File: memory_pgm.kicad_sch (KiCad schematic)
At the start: 14 parts

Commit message: Switch ROM chips to SRAM and add onboard programmer
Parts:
- removed J?: Conn_02x20_Odd_Even, symbol Connector_Generic:Conn_02x20_Odd_Even
- removed U? (x2): 28C256, symbol Memory_EEPROM:28C256
- removed U? (x4): 74HC245, symbol 74xx:74HC245
- removed U? (x5): 74LS32, symbol 74xx:74LS32
- added D? (x3): 1N4148, Diode_THT:D_DO-35_SOD27_P7.62mm_Horizontal, symbol Diode:1N4148
- added J?: QT Py RP2040, symbol Connector_Generic:Conn_02x07_Counter_Clockwise
- added J?: QT Py Serial, symbol Connector_Generic:Conn_01x03
- added R? (x6): 10K, symbol Device:R_Small_US
- added U? (x4): HEF4094BT, symbol parts:HEF4094BT
- added U? (x2): CY62256-70PC, Package_DIP:DIP-28_W15.24mm, symbol Memory_RAM:CY62256-70PC
- added U?: 74LS243, symbol 74xx:74LS243
- added U?: TXB0104PW, Package_SO:TSSOP-14_4.4x5mm_P0.65mm, symbol Logic_LevelTranslator:TXB0104PW
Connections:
- net A1: now also U?.10 (A0), U?.10 (A0), U?.4 (QP0)
- net A10: now also U?.24 (A9), U?.24 (A9), U?.5 (QP1)
- net A11: now also U?.21 (A10), U?.21 (A10), U?.6 (QP2)
- net A12: now also U?.23 (A11), U?.23 (A11), U?.7 (QP3)
- net A13: now also U?.14 (QP4), U?.2 (A12), U?.2 (A12)
- net A14: now also U?.13 (QP5), U?.26 (A13), U?.26 (A13)
- net A2: now also U?.5 (QP1), U?.9 (A1), U?.9 (A1)
- net A3: now also U?.6 (QP2), U?.8 (A2), U?.8 (A2)
- net A4: now also U?.7 (A3), U?.7 (A3), U?.7 (QP3)
- net A5: now also U?.14 (QP4), U?.6 (A4), U?.6 (A4)
- net A6: now also U?.13 (QP5), U?.5 (A5), U?.5 (A5)
- net A7: now also U?.12 (QP6), U?.4 (A6), U?.4 (A6)
- net A8: now also U?.11 (QP7), U?.3 (A7), U?.3 (A7)
- net A9: now also U?.25 (A8), U?.25 (A8), U?.4 (QP0)
- net D0: now also U?.11 (Q0), U?.4 (QP0)
- net D1: now also U?.12 (Q1), U?.5 (QP1)
- net D10: now also U?.13 (Q2), U?.6 (QP2)
- net D11: now also U?.15 (Q3), U?.7 (QP3)
- net D12: now also U?.14 (QP4), U?.16 (Q4)
- net D13: now also U?.13 (QP5), U?.17 (Q5)
- net D14: now also U?.12 (QP6), U?.18 (Q6)
- net D15: now also U?.11 (QP7), U?.19 (Q7)
- net D2: now also U?.13 (Q2), U?.6 (QP2)
- net D3: now also U?.15 (Q3), U?.7 (QP3)
- net D4: now also U?.14 (QP4), U?.16 (Q4)
- net D5: now also U?.13 (QP5), U?.17 (Q5)
- net D6: now also U?.12 (QP6), U?.18 (Q6)
- net D7: now also U?.11 (QP7), U?.19 (Q7)
- net D8: now also U?.11 (Q0), U?.4 (QP0)
- net D9: now also U?.12 (Q1), U?.5 (QP1)
- net GND: now also J?.13 (Pin_13), J?.3 (Pin_3), U?.1 (A14), U?.1 (A14), U?.14 (GND), U?.14 (GND), U?.5 (A4), U?.7 (GND), U?.7 (GND), U?.8 (B3), U?.8 (Vss), U?.8 (Vss), U?.8 (Vss), U?.8 (Vss)
- net VCC: now also R?.1, R?.1, R?.1, R?.1, R?.2, R?.2, U?.1 (OEa), U?.1 (STR), U?.1 (STR), U?.1 (STR), U?.1 (STR), U?.14 (VCC), U?.14 (VCCB), U?.16 (Vdd), U?.16 (Vdd), U?.16 (Vdd), U?.16 (Vdd), U?.28 (VCC), U?.28 (VCC)
- net ~{OE}: now also U?.22 (~{OE}), U?.22 (~{OE})
- net ~{ROMLDS}: now also U?.9 (B2)
- net ~{ROMUDS}: now also U?.10 (B1)
- net ~{WE}: now also U?.11 (B0); no longer U?.27 (~{WE}), U?.27 (~{WE})
- new net: R?.2, U?.12 (B2), U?.3 (CP), U?.3 (CP), U?.3 (CP), U?.3 (CP)
- new net: U?.10 (QS2), U?.2 (D) (x3)
- new net: D?.1 (K), D?.1 (K), D?.1 (K), R?.2, U?.10 (B4), U?.15 (~{OE}), U?.15 (~{OE}), U?.15 (~{OE}), U?.15 (~{OE})
- new net: J?.1 (Pin_1), U?.8 (OE)
- new net: J?.2 (Pin_2), U?.2 (A1)
- new net: J?.3 (Pin_3), U?.3 (A2)
- new net: J?.4 (Pin_4), U?.4 (A3)
- new net: J?.1 (Pin_1), J?.7 (Pin_7)
- new net: J?.2 (Pin_2), J?.8 (Pin_8)
- new net: R?.2, U?.13 (B1), U?.2 (D)
- new net +3V3: J?.12 (Pin_12), U?.1 (VCCA)
- new net ~{RESET}: D?.2 (A), U?.13 (OEb)
- new net ~{ROMLDS_INT}: D?.2 (A), R?.1, U?.20 (~{CS}), U?.5 (A2)
- new net ~{ROMUDS_INT}: D?.2 (A), R?.1, U?.20 (~{CS}), U?.4 (A1)
- new net ~{WE_INT}: R?.2, U?.11 (B3), U?.27 (~{WE}), U?.27 (~{WE}), U?.27 (~{WE}), U?.27 (~{WE}), U?.3 (A0)
- no-connect marks 2 -> 14
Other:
- moved on the sheet: U?

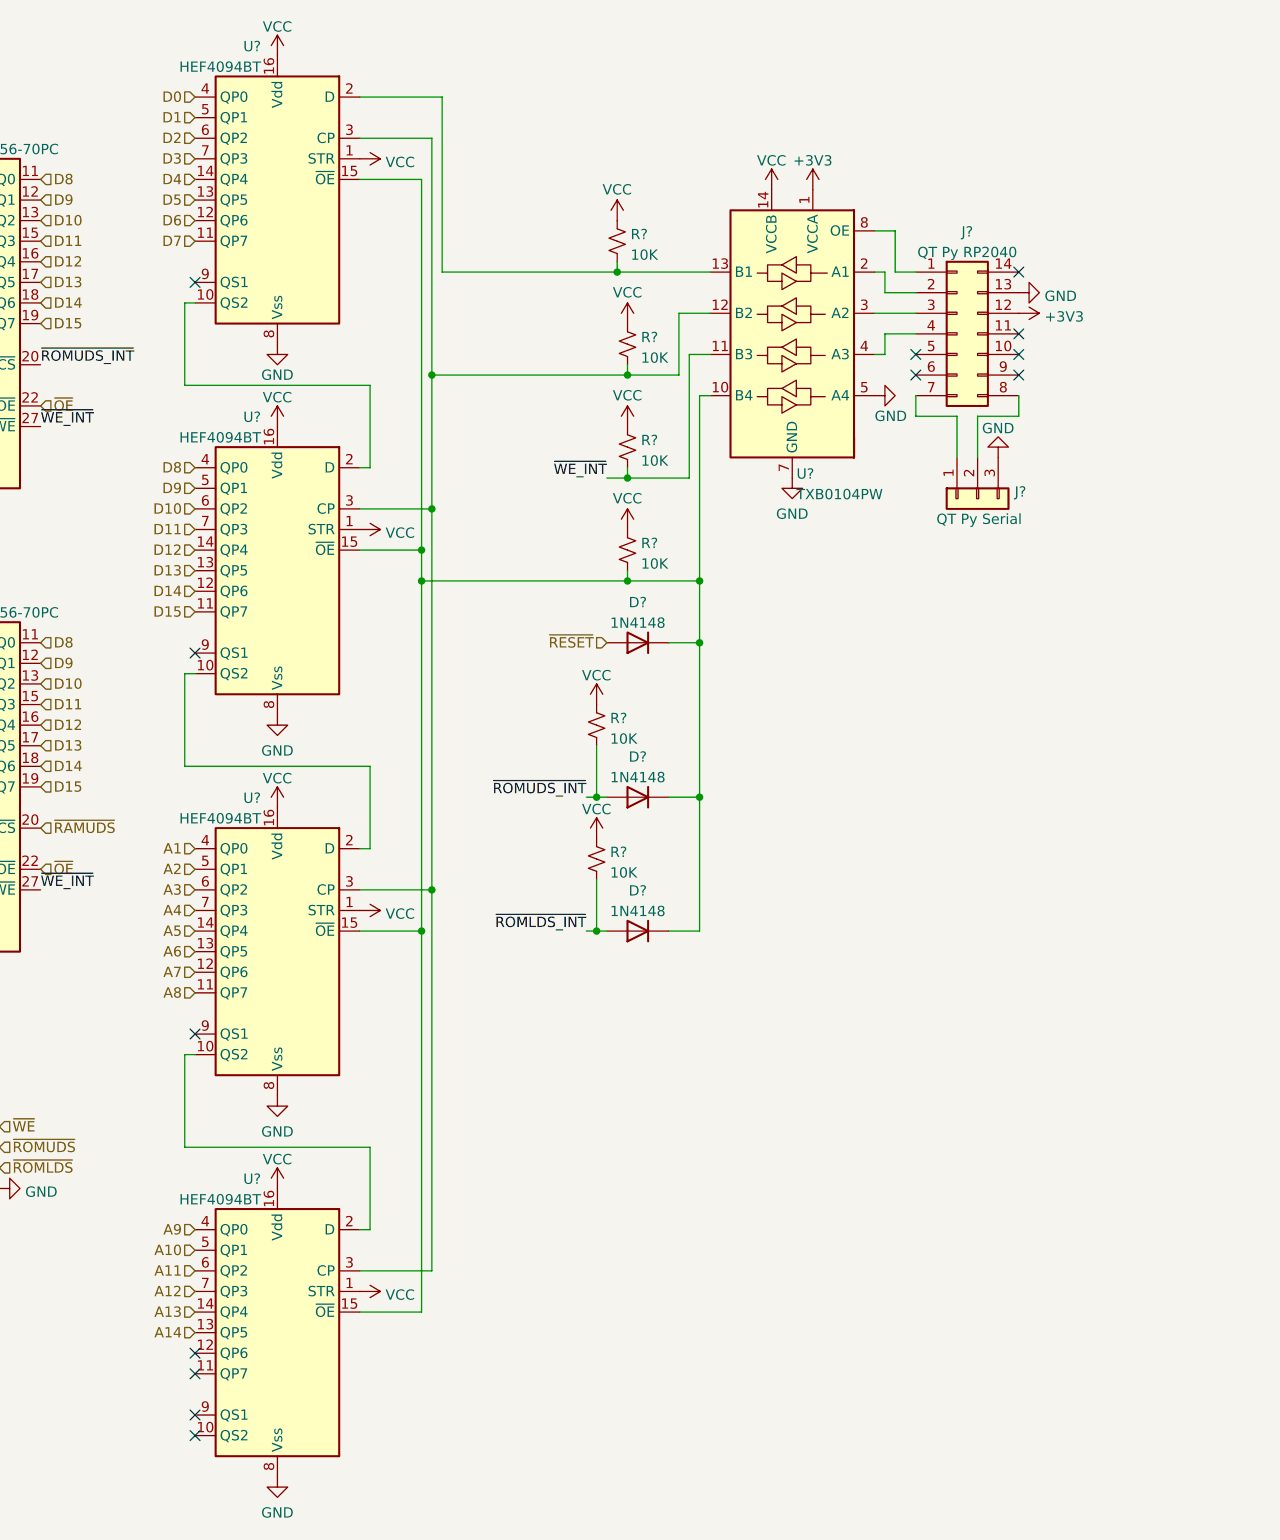
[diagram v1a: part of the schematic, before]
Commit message: Add title and rev number
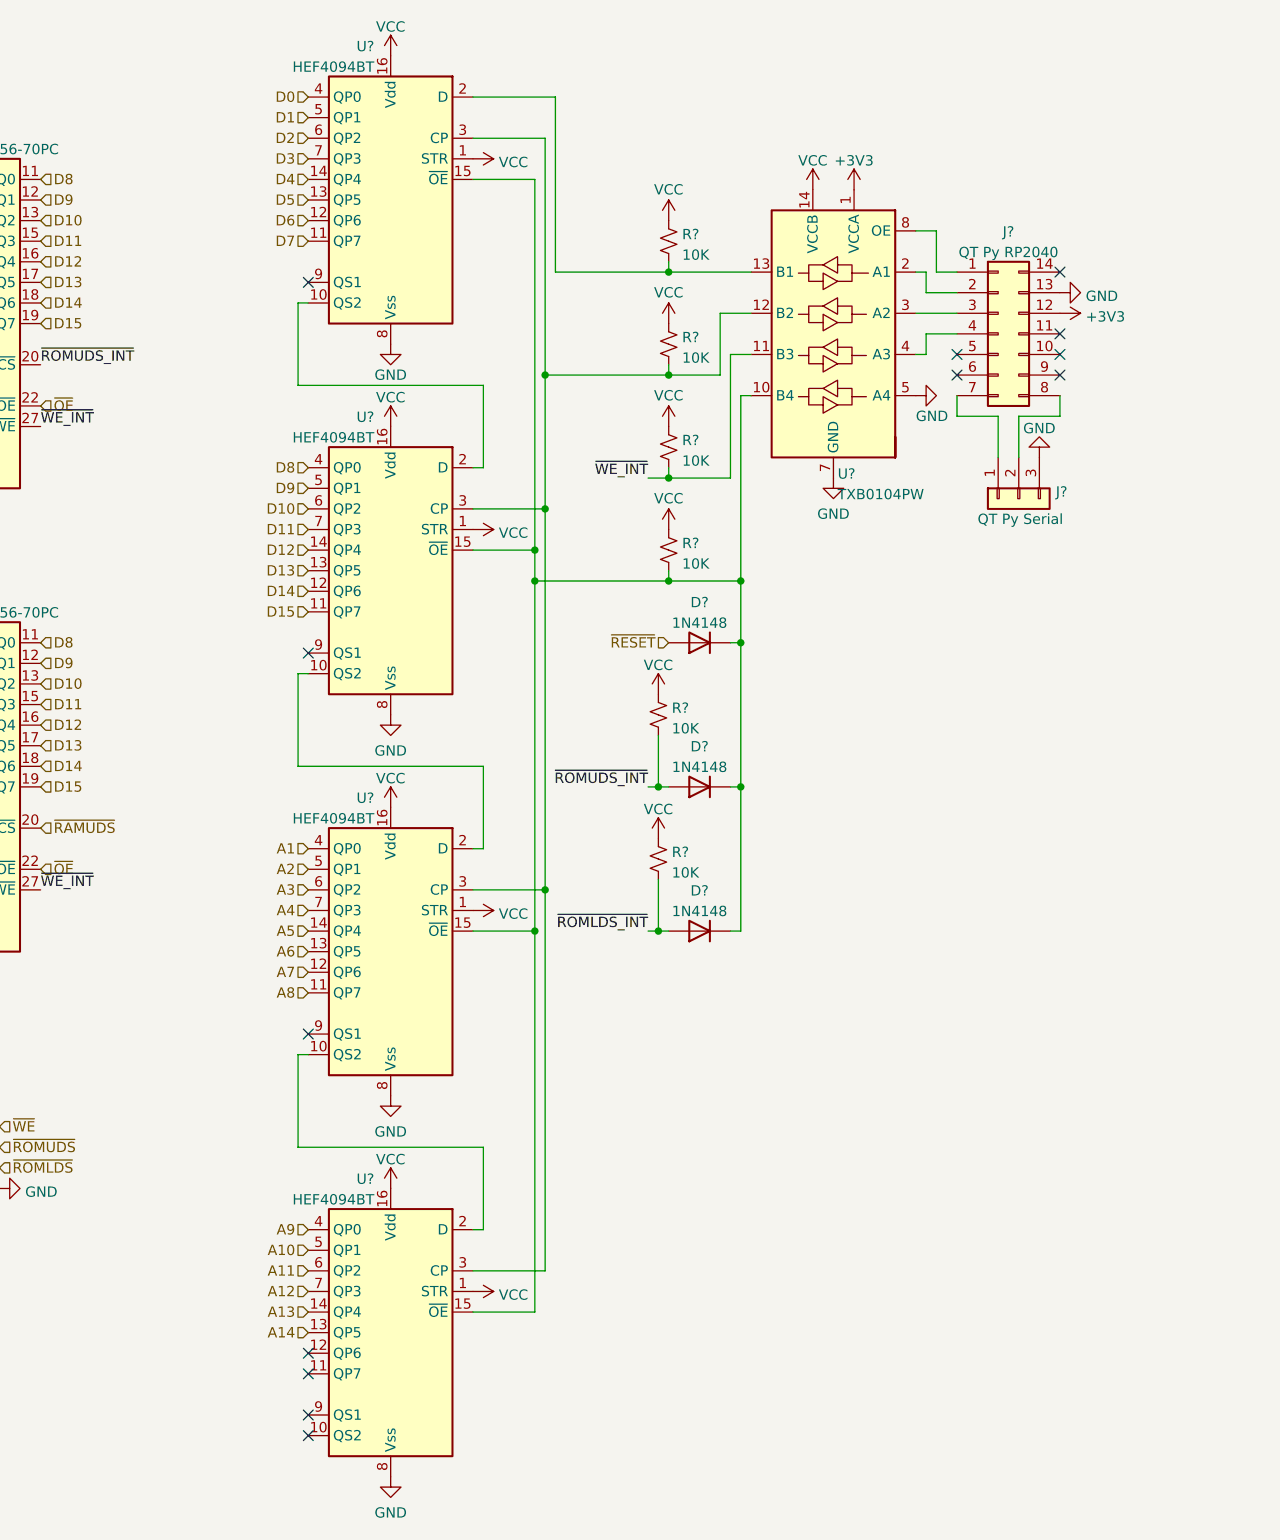
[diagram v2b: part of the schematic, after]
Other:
- title: (none) -> RAM/ROM Board
- moved on the sheet: D?, J?, R?, U?
